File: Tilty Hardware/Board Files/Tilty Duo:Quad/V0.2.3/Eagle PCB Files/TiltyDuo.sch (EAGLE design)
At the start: 44 parts, among them U1 TEENSY_3.0_OUTER-PINS28-DIP_S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, U2 HC-09_BREAKOUT, U3 MPL3115A2LGA8, U4 LM2931, U5 MPU-6050, U6 HMC5883LSMD, U7 SPI_FLASH-X25XXSMD

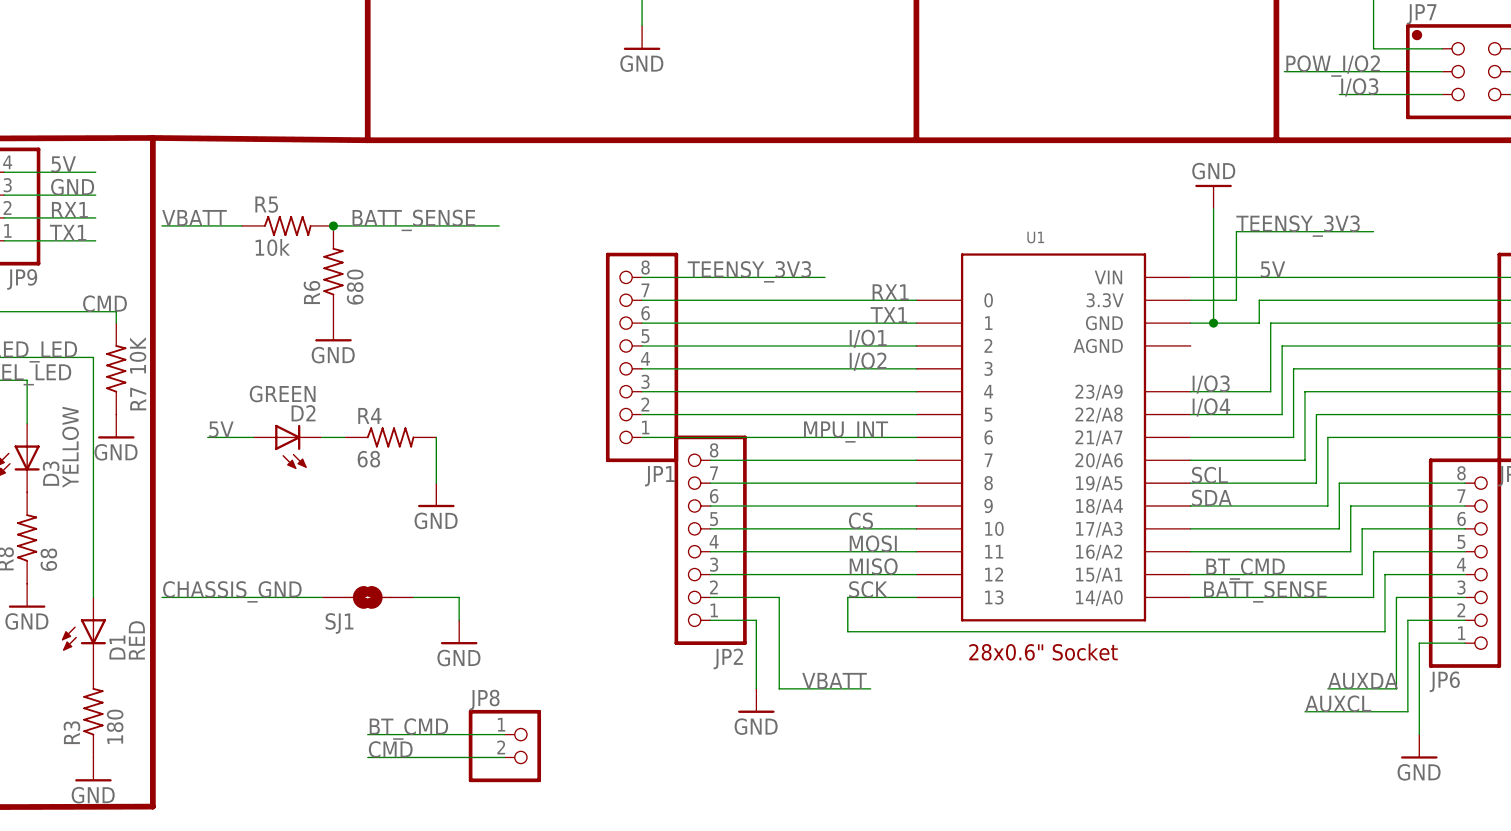
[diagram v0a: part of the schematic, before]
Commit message: Lots of little tweaks to perfect the Tilty Duo/Quad and updated ToDo list
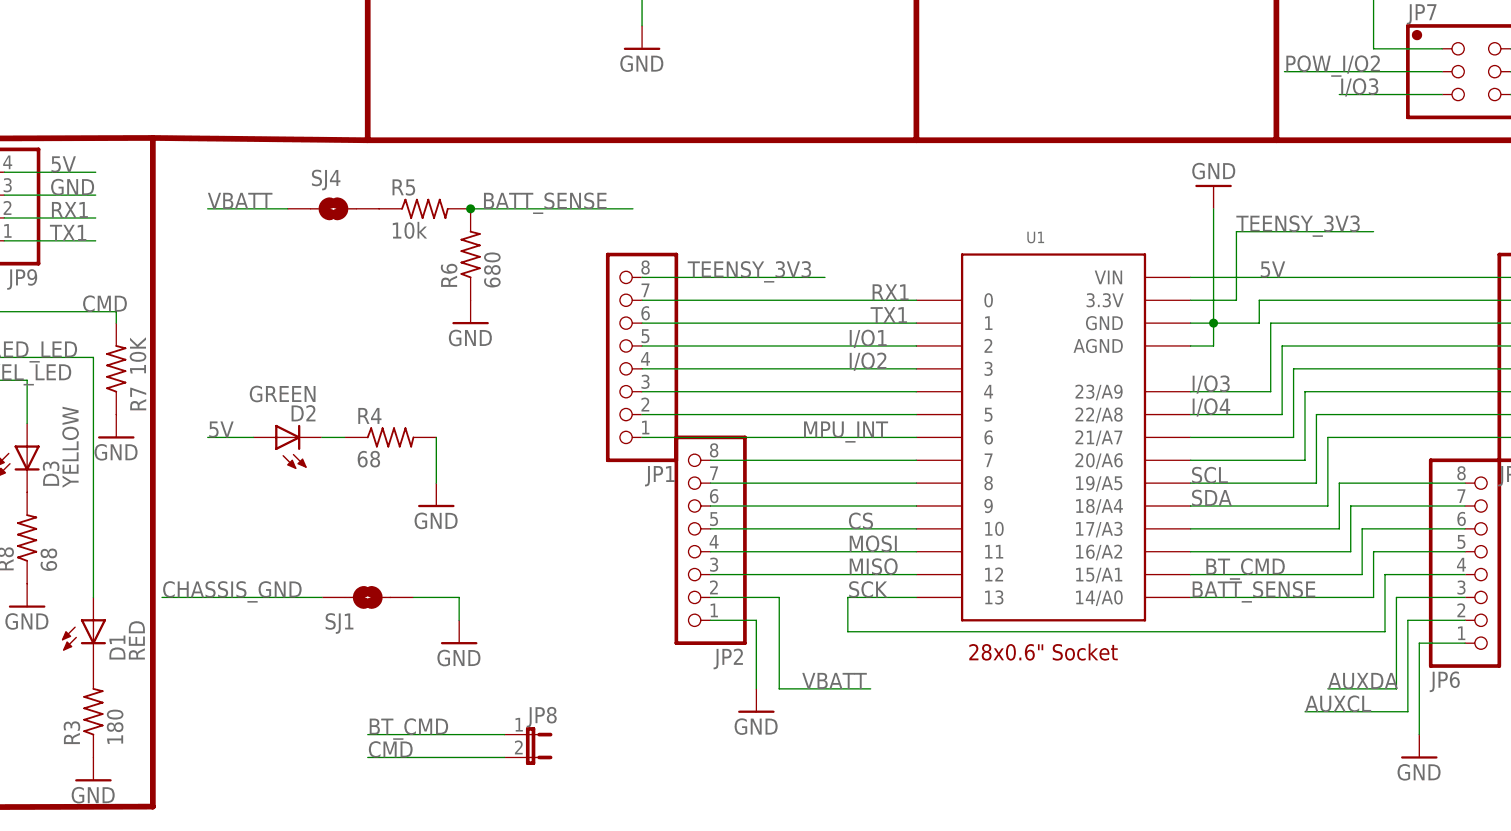
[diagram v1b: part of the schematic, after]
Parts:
- added SJ4: SOLDERJUMPERTRACE, SparkFun-Passives:SOLDERJUMPERTRACE
- JP8: device pinhead:PINHD-1X21X02_NO_SILK -> SparkFun-Passives:JUMPER-2SMD-NC
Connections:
- new net N$9: R5.1, SJ4.2
- net GND: now also U1.AGND
- net VBATT: now also SJ4.1; no longer R5.1
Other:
- moved on the sheet: R5, R6
